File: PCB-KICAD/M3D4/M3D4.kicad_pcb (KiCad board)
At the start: 2 copper layers, 76 x 31 mm, 29 parts, among them J1 USB_B, P2 STDCONN, U1 CM108AH, U4 93CxxA, U5 AMS1117-5.0, U6 AMS1117-3.3, Y1 12MHz

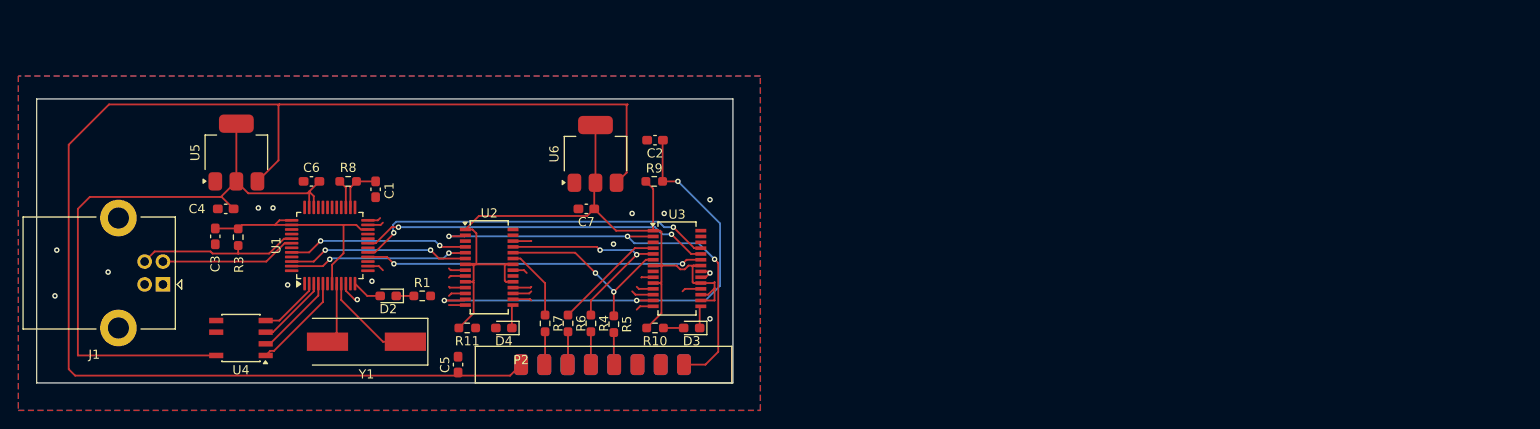
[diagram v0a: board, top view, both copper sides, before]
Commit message: First test board.
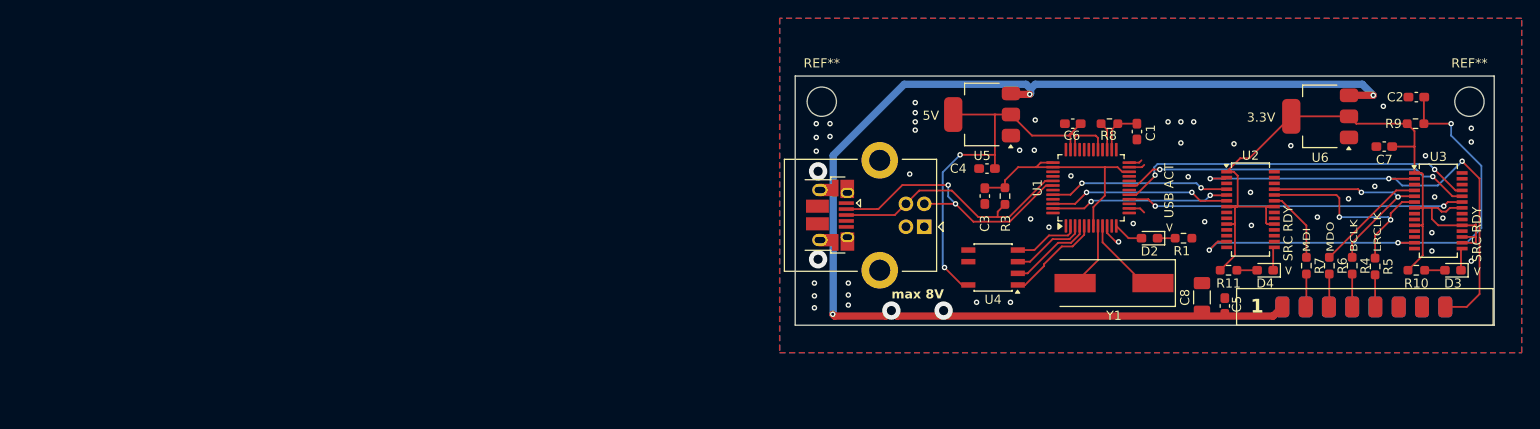
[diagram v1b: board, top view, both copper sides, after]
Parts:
- added C8: 10u, Capacitor_SMD:C_1206_3216Metric_Pad1.33x1.80mm_HandSolder, F.Cu at (148.2, 93.2)
- added J2: USB_B_Micro, Connector_USB:USB_Micro-B_Amphenol_10103594-0001LF_Horizontal, F.Cu at (107.6, 84.2)
- added REF**: MountingHole_3.2mm_M3, MountingHole:MountingHole_3.2mm_M3, F.Cu at (177.4, 71.8)
- added REF**: MountingHole_3.2mm_M3, MountingHole:MountingHole_3.2mm_M3, F.Cu at (106.7, 71.8)
- moved C7 87.4 mm to (168.1, 76.7)
- moved C3 84.1 mm to (124.5, 82.1)
- moved C5 83.9 mm to (150.7, 94.1)
- moved R3 83.8 mm to (126.7, 82.1)
- moved C1 83.3 mm to (141.1, 75.1)
- moved C6 83.3 mm to (134.1, 74.2)
- moved D2 83.3 mm to (142.5, 86.7)
- moved D3 83.3 mm to (175.6, 90.2)
- moved D4 83.3 mm to (155.1, 90.2)
- moved J1 83.3 mm to (117.9, 85.5)
- moved P2 83.3 mm to (157.0, 94.2)
- moved R1 83.3 mm to (146.2, 86.7)
- moved R10 83.3 mm to (171.6, 90.2)
- moved R11 83.3 mm to (151.1, 90.2)
- moved R4 83.3 mm to (164.6, 89.7)
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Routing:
- net GND: track 38.5 -> 7.43 mm, vias 14 -> 50
- net +5V: track 71.7 -> 49.4 mm, vias 0 -> 2
- net VIN: track 155.9 -> 135.9 mm, vias 0 -> 5
- net Net-(J1-D-): track 14.9 -> 31.1 mm, vias 0 -> 2
- net Net-(J1-D+): track 18.1 -> 28.2 mm
- net +3.3V: track 91.2 -> 85.5 mm
- net MCLK: track 49.3 -> 53.2 mm
- net Net-(U2-LRCKO): track 21.2 -> 23.7 mm
- net Net-(D4-A): track 0.00 -> 2.21 mm
- net Net-(U1-XO): track 10.7 -> 9.13 mm
- net RST: track 54.4 -> 53.4 mm
- net Net-(U1-XI): track 6.75 -> 7.27 mm
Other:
- board size 76 x 31 mm -> 76.3 x 27.2 mm
- board text added: "1"
- board text added: "2"
- board text added: "3.3V"
- board text added: "5V"
- board text added: "< SRC RDY"
- board text added: "< USB ACT"
- board text added: "@mb 2024"
- board text added: "FreeDSP-USB-IO"
- board text added: "MDI MDO BCLK LRCLK"
- board text added: "freedsp con"
- board text added: "max 8V"
